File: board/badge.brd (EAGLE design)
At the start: 157.3 x 91.3 mm, 47 parts, among them IC1 STM32F030F4, IC2 UBLOX_MAX, IC3 MCP1640, IC4 RFM69HW, J1 SWD_PTH_SHROUD, X1 SMA-142-0701-851/861, X2 1503_02, X3 091OLED, X4 RADIOMETRIX-MTX2

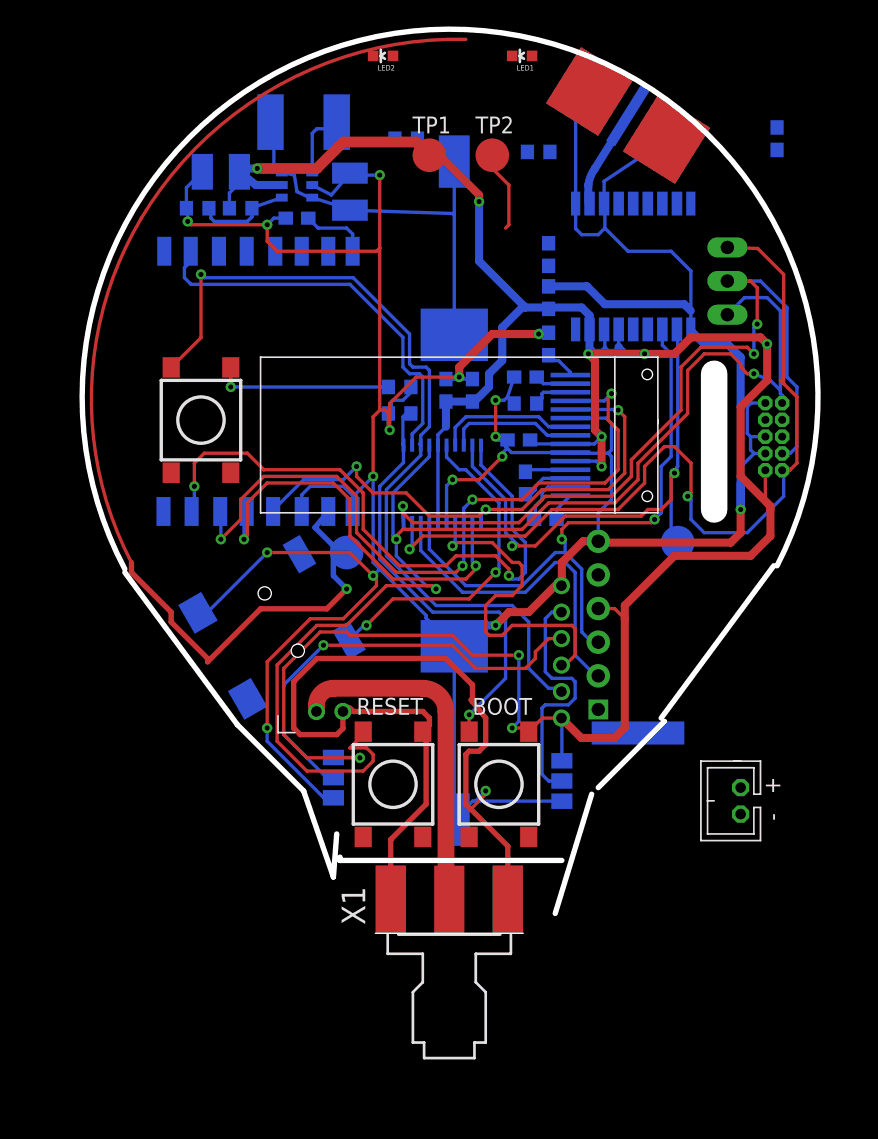
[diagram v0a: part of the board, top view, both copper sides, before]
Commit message: almost done
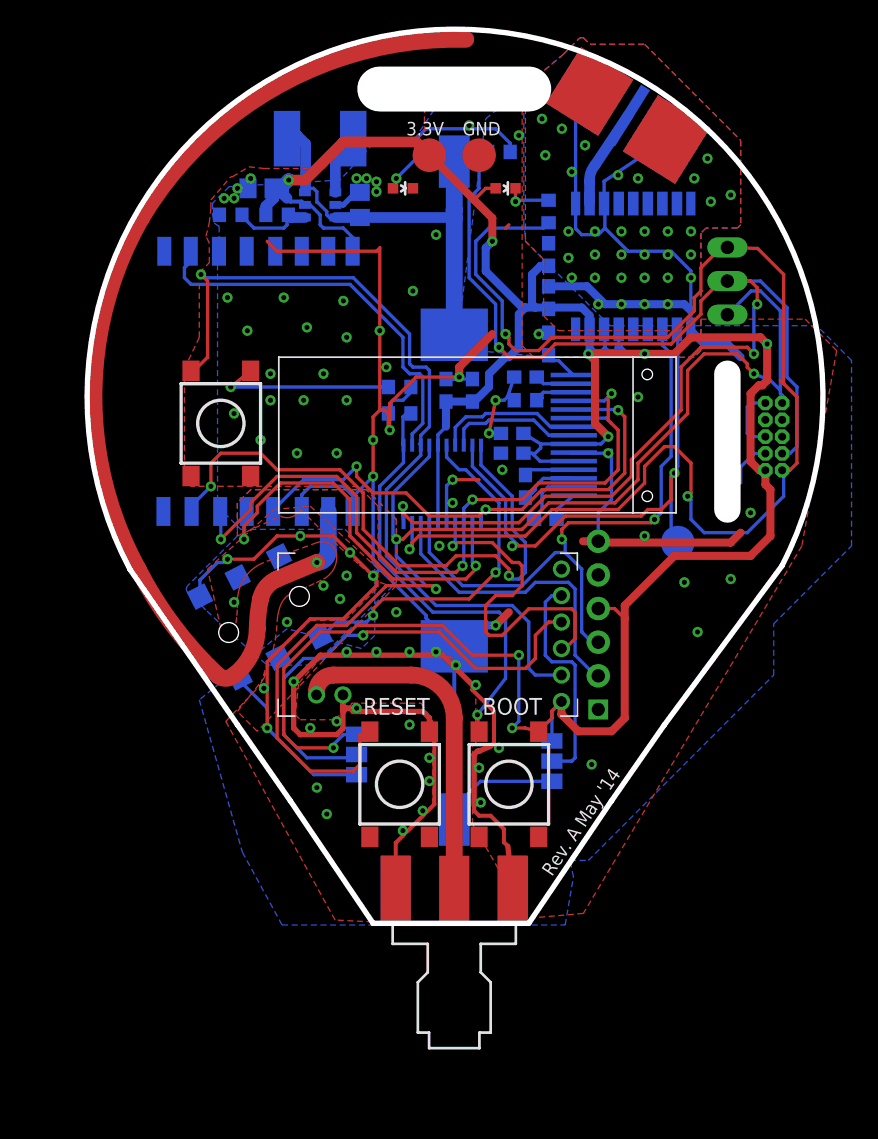
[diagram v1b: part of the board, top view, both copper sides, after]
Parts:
- removed C13: 1u, rcl:C0603
- removed TP4: PTR1B2,54, testpad:B2,54
- removed U$4: INDUCTOR, ukhas:INDUCTOR5X5
- removed U$6: (no value), ukhas:0.91OLEDPANEL
- removed X4: RADIOMETRIX-MTX2, Ava:RADIOMETRIX-MTX2
- added L1: INDUCTOR, ukhas:INDUCTOR5X5
- added U$1: (no value), ukhas:0.91OLEDPANEL
- C1, C2, C4: value (none) -> 1u
- C11, C12: value 2u2 -> (none); device rcl:C0603 -> rcl:C0805
- C5, C6: value 1u -> (none)
- C7, C8: value (none) -> 2u2; device rcl:C1210 -> rcl:C0603
- IC3: value MCP1640 -> RFM69HW; device ukhas:SOT23-6 -> hoperf:RFM
- IC4: value RFM69HW -> MCP1640; device hoperf:RFM -> ukhas:SOT23-6
- J2: value (none) -> 20-0096; device dtb:JST-2-TH -> ukhas:3.5MMLOWPROFILE
- R3: value (none) -> 1k
- R7: value 1k -> (none)
- X1: value SMA-142-0701-851/861 -> RADIOMETRIX-MTX2; device con-coax:J502-ND-142-0701-851/861 -> Ava:RADIOMETRIX-MTX2
- X2: value 1503_02 -> SMA-142-0701-851/861; device con-lumberg:1503_02 -> con-coax:J502-ND-142-0701-851/861
- moved J2 44.6 mm to (12.0, 37.2), flipped to the bottom, turned to 153 degrees
- moved S3 36.0 mm to (36.8, 24.2)
- moved S1 30.2 mm to (15.0, 51.5)
- moved C8 28.0 mm to (39.8, 57.5), turned to 270 degrees
- moved X2 27.1 mm to (32.6, 13.8), flipped to the top, turned to 90 degrees
- moved R2 25.9 mm to (38.0, 53.2), turned to 180 degrees
- moved C12 24.6 mm to (18.0, 69.2)
- moved R5 23.7 mm to (15.8, 67.2)
- moved R4 23.6 mm to (19.2, 67.2), turned to 0 degrees
- moved X1 22.8 mm to (30.8, 35.8), turned to 0 degrees
- moved R3 20.4 mm to (28.5, 54.2)
- moved C9 19.9 mm to (39.8, 61.0), turned to 90 degrees
- moved C10 19.3 mm to (39.8, 64.2), turned to 90 degrees
- moved C7 19.3 mm to (38.0, 55.0), turned to 0 degrees
- moved R7 19.3 mm to (36.0, 72.0), turned to 0 degrees
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- renumbered B2 to B1, J1 to J3, U$5 to U$2
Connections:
- net +3V3: now also C12.1, C4.2, C5.1, C6.1, IC3.VCC, IC4.5, LED2.A, R4.2, S3.A2, X1.VCC; no longer C1.1, C13.2, C2.1, C4.1, C8.1, IC3.5, IC4.VCC, LED1.A, R2.2, S2.A2, X4.VCC
- net 0V: now also C11.2, C4.1, C5.2, C6.2, C8.1, IC3.GNDA, IC3.GNDB, IC4.2, J2.2_1, J2.2_2, LED1.C, R2.1, R3.2, R5.1, S2.A2, X1.GND, X1.RFGND, X2.G@1, X2.G@2, X2.G@3, X2.G@4; no longer C1.2, C11.1, C13.1, C2.2, C4.2, C8.2, IC3.2, IC4.GNDA, IC4.GNDB, LED2.C, R3.1, R4.1, R7.2, S1.A2, X1.G@1, X1.G@2, X1.G@3, X1.G@4, X2.2, X4.GND, X4.RFGND
- net ADC1: now also J2.4_1, J2.4_2; no longer X2.3
- net CS: now also IC3.NSS; no longer IC4.NSS
- net DIO0: now also IC3.DIO0; no longer IC4.DIO0
- net MISO: now also IC3.MISO; no longer IC4.MISO
- net MOSI: now also IC3.MOSI; no longer IC4.MOSI
- net N$10: now also C2.2; no longer C5.2
- net N$11: now also C1.2; no longer C6.2
- net N$12: now also C2.1; no longer C5.1
- net N$13: now also C1.1; no longer C6.1
- net N$14: now also IC4.4, R4.1, R5.2; no longer IC3.4, R2.1, R3.2
- net N$15: now also IC4.1, L1.P$2; no longer IC3.1, U$4.P$2
- net N$16: now also C7.1; no longer C12.1
- net N$17: now also LED1.A, R7.1; no longer LED2.A, R6.1
- net N$18: now also X1.P1; no longer X4.P1
- net N$19: now also R3.1, S1.A2; no longer R7.1, S3.A2
- net N$20: now also X1.P0; no longer X4.P0
- net N$3: now also LED2.C, R6.2; no longer LED1.C, R5.2
- net N$4: now also X1.RF, X2.1; no longer X1.1, X4.RF
- net N$5: now also R2.2; no longer R4.2
- net N$6: now also IC3.ANT; no longer IC4.ANT, TP4.TP
- net N$7: now also S3.B2; no longer S2.B2
- net NRST: now also S2.B2; no longer S1.B2
- net SCK: now also IC3.SCK; no longer IC4.SCK
- net SWCLK: now also R7.2; no longer R6.2
- net SWDAT: now also R6.1; no longer R5.1
- net TX: now also X1.TXD; no longer X4.TXD
- net TX_EN: now also S1.B2, X1.EN; no longer S3.B2, X4.EN
- net VCC: now also C8.2; no longer C11.2
- net VIN: now also C11.1, IC4.3, IC4.6, L1.P$1; no longer C7.1, IC3.3, IC3.6, U$4.P$1
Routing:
- net 0V: track 380.8 -> 318.4 mm, vias 17 -> 114
- net SWCLK: track 61.9 -> 98.9 mm, vias 3 -> 4
- net SWDAT: track 64.3 -> 101.0 mm, vias 2 -> 3
- net N$17: track 0.00 -> 13.0 mm, vias 0 -> 1
- net N$18: track 33.0 -> 36.6 mm
- net N$3: track 0.00 -> 3.54 mm, vias 0 -> 1
- net N$6: track 83.8 -> 81.3 mm
- net ADC1: track 24.8 -> 27.2 mm
- net +3V3: track 207.0 -> 209.0 mm, vias 10 -> 9
- net N$20: track 18.8 -> 16.8 mm
- net N$9: track 25.0 -> 23.1 mm
- net NRST: track 97.8 -> 96.2 mm
- net N$4: track 25.8 -> 26.7 mm
- net MOSI: track 55.1 -> 54.3 mm
- net N$14: track 7.21 -> 6.39 mm
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- added copper zone on layer 1, net 0V
- added copper zone on layer 16, net 0V
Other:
- board size 157.3 x 91.3 mm -> 157.7 x 91.3 mm
- board text added: "0"
- board text added: "1"
- board text added: "3.3V"
- board text added: "GND"
- board text added: "GPS TX"
- board text added: "P0"
- board text added: "P1"
- board text added: "Rev. A May '14"
